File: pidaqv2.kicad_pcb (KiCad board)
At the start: 2 copper layers, 81.3 x 71.1 mm, 28 parts, among them J101 Conn_02x04_Odd_Even, J102 Conn_01x03, J103 Screw_Terminal_01x10, J104 Screw_Terminal_01x08, J105 Screw_Terminal_01x06, J106 Screw_Terminal_01x08, J107 Conn_01x03_Male, U101 INA2126E_250, U201 ADS1261BIRHBR, U301 ADS1261BIRHBR

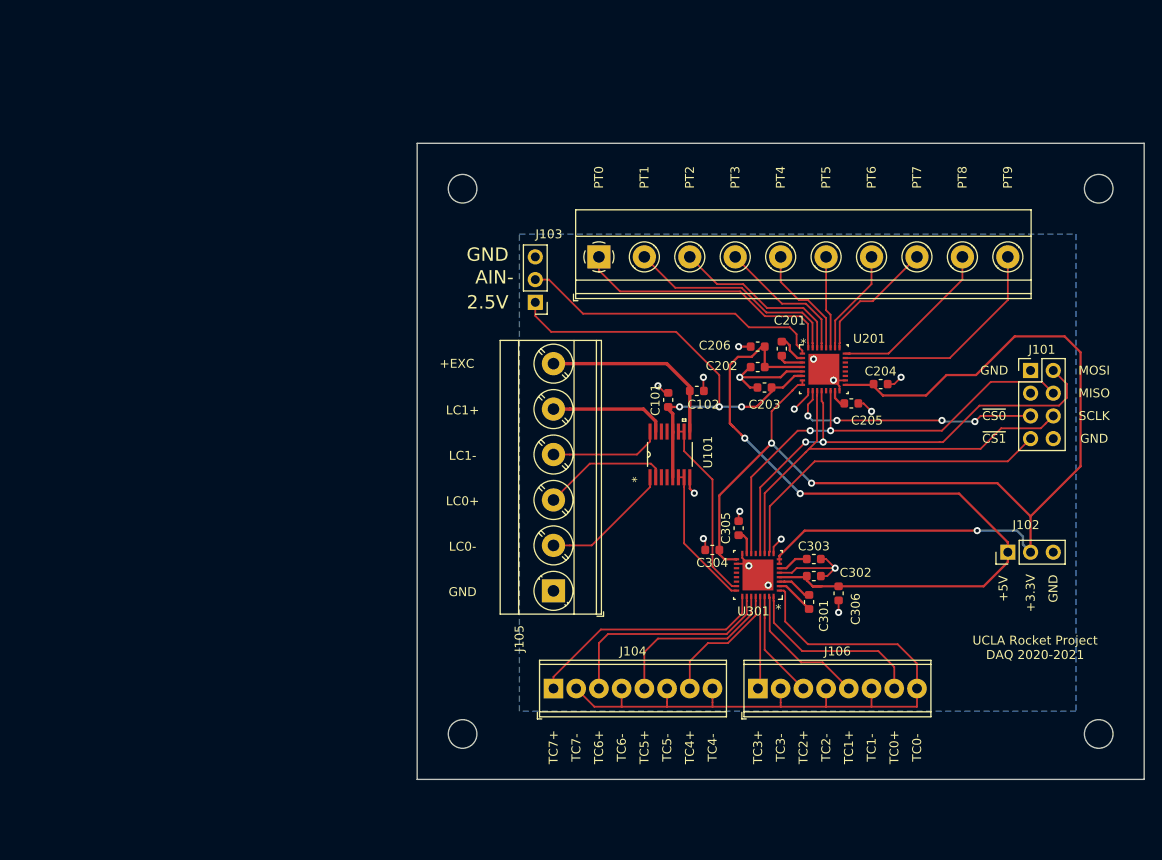
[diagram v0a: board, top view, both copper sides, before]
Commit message: boi did i cut up that ground plane
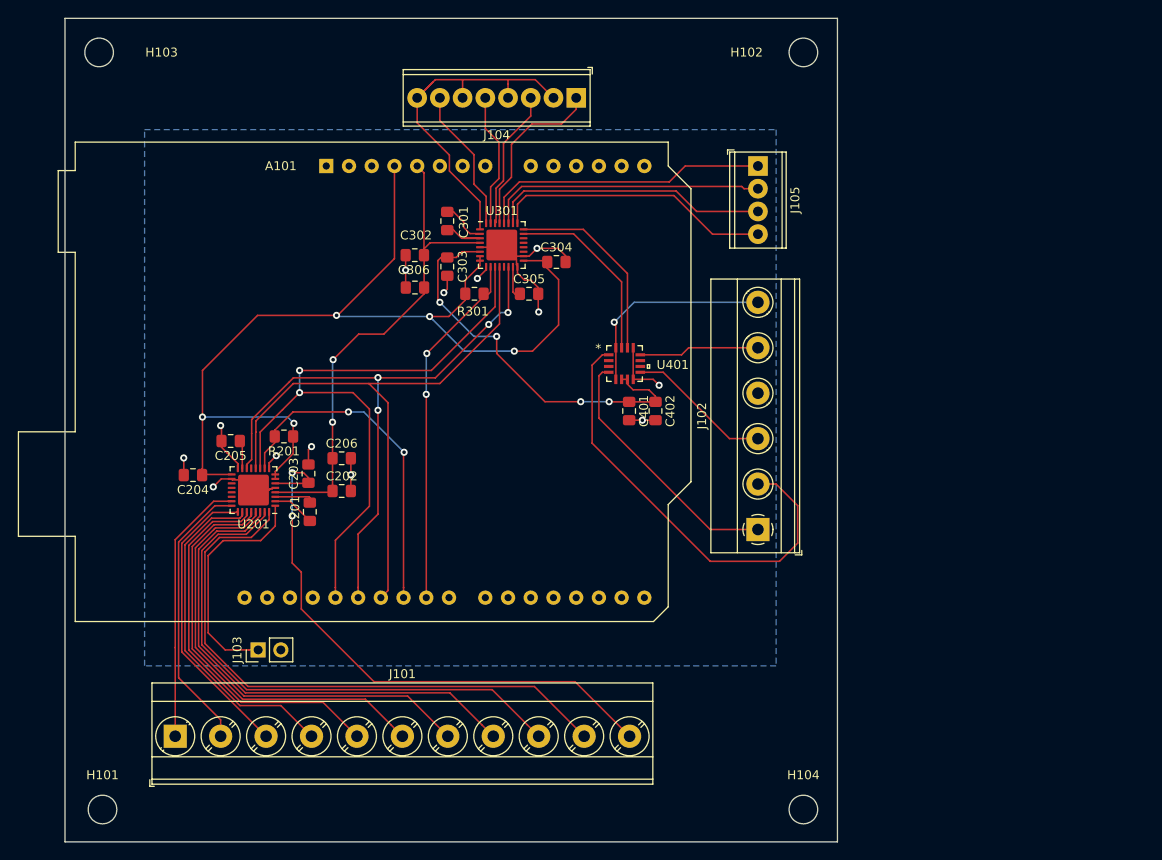
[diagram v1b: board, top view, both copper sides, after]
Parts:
- removed C101, C102: 0.1uF, Capacitor_SMD:C_0603_1608Metric
- removed J106: Screw_Terminal_01x08, TerminalBlock_Phoenix:TerminalBlock_Phoenix_MPT-0,5-8-2.54_1x08_P2.54mm_Horizontal
- removed J107: Conn_01x03_Male, Connector_PinHeader_2.54mm:PinHeader_1x03_P2.54mm_Vertical
- removed U101: INA2126E_250, footprints:INA2126E&slash_250
- added A101: Arduino_UNO_R3, Module:Arduino_UNO_R3, F.Cu at (86.4, 71.1)
- added C401: 0.1uF, Capacitor_SMD:C_0805_2012Metric_Pad1.15x1.40mm_HandSolder, F.Cu at (120.2, 98.5)
- added C402: 10uF, Capacitor_SMD:C_0805_2012Metric_Pad1.15x1.40mm_HandSolder, F.Cu at (123.2, 98.5)
- added R201: 4.7K, Resistor_SMD:R_0805_2012Metric_Pad1.15x1.40mm_HandSolder, F.Cu at (81.6, 101.4)
- added R301: 4.7K, Resistor_SMD:R_0805_2012Metric_Pad1.15x1.40mm_HandSolder, F.Cu at (102.9, 85.4)
- added U401: AD8426ACPZ-R7, footprints:AD8426ACPZ-R7, F.Cu at (119.7, 93.2)
- C201, C202, C203, C204, C205, C206, C301, C302, C303, C304, C305, C306: footprint Capacitor_SMD:C_0603_1608Metric -> Capacitor_SMD:C_0805_2012Metric_Pad1.15x1.40mm_HandSolder
- J101: value Conn_02x04_Odd_Even -> Screw_Terminal_01x11; footprint Connector_PinHeader_2.54mm:PinHeader_2x04_P2.54mm_Vertical -> TerminalBlock_Phoenix:TerminalBlock_Phoenix_MKDS-3-11-5.08_1x11_P5.08mm_Horizontal
- J102: value Conn_01x03 -> Screw_Terminal_01x06; footprint Connector_PinHeader_2.54mm:PinHeader_1x03_P2.54mm_Vertical -> TerminalBlock_Phoenix:TerminalBlock_Phoenix_MKDS-1,5-6-5.08_1x06_P5.08mm_Horizontal
- J103: value Screw_Terminal_01x10 -> Conn_01x02_Male; footprint TerminalBlock_Phoenix:TerminalBlock_Phoenix_MKDS-1,5-10-5.08_1x10_P5.08mm_Horizontal -> Connector_PinHeader_2.54mm:PinHeader_1x02_P2.54mm_Vertical
- J105: value Screw_Terminal_01x06 -> Screw_Terminal_01x04; footprint TerminalBlock_Phoenix:TerminalBlock_Phoenix_MKDS-3-6-5.08_1x06_P5.08mm_Horizontal -> TerminalBlock_Phoenix:TerminalBlock_Phoenix_MPT-0,5-4-2.54_1x04_P2.54mm_Horizontal
- U201, U301: footprint footprints:ADS1261BIRHBR -> Package_DFN_QFN:Texas_S-PVQFN-N32_EP3.45x3.45mm
- moved H103 112.8 mm to (61.0, 58.4)
- moved H101 111.7 mm to (61.3, 143.1)
- moved J101 104.0 mm to (69.5, 134.9)
- moved H102 85.2 mm to (139.7, 58.4)
- moved H104 79.2 mm to (139.7, 143.1)
- moved C204 77.6 mm to (71.5, 105.7), turned to 180 degrees
- moved C205 69.5 mm to (75.7, 101.9), turned to 180 degrees
- moved J104 66.1 mm to (114.3, 63.5), turned to 180 degrees
- moved U201 65.2 mm to (78.2, 107.4), turned to 180 degrees
- moved C301 58.7 mm to (99.9, 77.3), turned to 270 degrees
- moved C306 58.4 mm to (96.3, 84.7), turned to 180 degrees
- moved J103 58.2 mm to (78.7, 125.2), turned to 90 degrees
- moved C302 57.2 mm to (96.3, 81.1), turned to 180 degrees
- moved C201 55.8 mm to (84.5, 109.8), turned to 90 degrees
- moved J105 52.7 mm to (134.6, 71.1), turned to 270 degrees
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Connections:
- net TC- renamed /ADC1/AINCOM
- C203 pad 1: 2.5V -> /ADC0/REF2.5V
- J101 pad 1: GND -> /ADC0/AIN9
- J101 pad 2: MOSI -> /ADC0/AIN8
- J101 pad 3: (no net) -> /ADC0/AIN7
- J101 pad 4: MISO -> /ADC0/AIN6
- J101 pad 5: ~CS0 -> /ADC0/AIN5
- J101 pad 6: SCLK -> /ADC0/AIN4
- J101 pad 7: ~CS1 -> /ADC0/AIN3
- J101 pad 8: GND -> /ADC0/AIN2
- J102 pad 1: +5V -> /amplifier/A+
- J102 pad 2: +3V3 -> /amplifier/A-
- J102 pad 3: GND -> /amplifier/B+
- J103 pad 1: /ADC0/AIN0 -> /ADC0/AINCOM
- J103 pad 2: /ADC0/AIN1 -> GND
- J104 pad 1: (no net) -> /ADC1/AIN3
- J104 pad 3: TC6 -> /ADC1/AIN2
- J104 pad 5: TC5 -> /ADC1/AIN1
- J104 pad 7: TC4 -> /ADC1/AIN0
- J105 pad 1: GND -> /ADC1/AIN4
- J105 pad 2: LC0- -> /ADC1/AIN5
- J105 pad 3: LC0+ -> /ADC1/AIN6
- J105 pad 4: LC1- -> /ADC1/AIN7
- U201 pad 1: /ADC0/AIN- -> /ADC0/AINCOM
- U201 pad 6: 2.5V -> /ADC0/REF2.5V
- U301 pad 23: LC1 -> /A
- U301 pad 24: LC0 -> /B
- U301 pad 25: (no net) -> /ADC1/AIN7
- U301 pad 26: TC6 -> /ADC1/AIN6
- U301 pad 27: TC5 -> /ADC1/AIN5
- U301 pad 28: TC4 -> /ADC1/AIN4
- U301 pad 29: TC3 -> /ADC1/AIN3
- U301 pad 30: TC2 -> /ADC1/AIN2
- U301 pad 31: TC1 -> /ADC1/AIN1
- U301 pad 32: TC0 -> /ADC1/AIN0
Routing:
- net /ADC0/REF2.5V: track 0.00 -> 64.6 mm, vias 0 -> 2
- net 2.5V: track 53.5 -> 0.00 mm, vias 3 -> 0
- net /amplifier/A-: track 0.00 -> 50.0 mm
- net /ADC1/REF2.5V: track 3.49 -> 45.2 mm, vias 0 -> 4
- net /ADC0/AIN1: track 24.7 -> 61.5 mm
- net /ADC0/AIN2: track 20.2 -> 56.8 mm
- net /ADC0/AIN0: track 30.0 -> 66.5 mm
- net /ADC0/AIN3: track 15.7 -> 52.1 mm
- net /ADC1/AINCOM: track 76.7 -> 41.1 mm
- net /ADC0/AIN4: track 12.9 -> 47.9 mm
- net /ADC0/AIN-: track 34.2 -> 0.00 mm
- net /ADC1/AIN4: track 0.00 -> 32.7 mm
- net /ADC0/AIN5: track 10.4 -> 42.8 mm
- net /ADC1/AIN6: track 0.00 -> 31.7 mm
- net /ADC1/AIN5: track 0.00 -> 31.2 mm
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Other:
- board size 81.3 x 71.1 mm -> 86.4 x 92.1 mm
- net class Default: clearance 0.2032 -> 0.1778; trace_width 0.2032 -> 0.1778
- rule trace_clearance: 0.2032 -> 0.1778
- rule trace_min: 0.2032 -> 0.1524
- board text removed: "+3.3V"
- board text removed: "+5V"
- board text removed: "+EXC"
- board text removed: "2.5V"
- board text removed: "AIN-"
- board text removed: "GND"
- board text removed: "LC0+"
- board text removed: "LC0-"
- board text removed: "LC1+"
- board text removed: "LC1-"
- board text removed: "MISO"
- board text removed: "MOSI"
- board text removed: "PT0"
- board text removed: "PT1"
- board text removed: "PT2"
- board text removed: "PT3"
- board text removed: "PT4"
- board text removed: "PT5"
- board text removed: "PT6"
- board text removed: "PT7"
- board text removed: "PT8"
- board text removed: "PT9"
- board text removed: "Raspi mounted here"
- board text removed: "SCLK"
- board text removed: "TC0+"
- board text removed: "TC0-"
- board text removed: "TC1+"
- board text removed: "TC1-"
- board text removed: "TC2+"
- board text removed: "TC2-"
- board text removed: "TC3+"
- board text removed: "TC3-"
- board text removed: "TC4+"
- board text removed: "TC4-"
- board text removed: "TC5+"
- board text removed: "TC5-"
- board text removed: "TC6+"
- board text removed: "TC6-"
- board text removed: "TC7+"
- board text removed: "TC7-"
- board text removed: "UCLA Rocket Project DAQ 2020-2021"
- board text removed: "~CS0"
- board text removed: "~CS1"
